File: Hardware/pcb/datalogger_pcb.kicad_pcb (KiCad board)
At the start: 2 copper layers, 123 x 86 mm, 45 parts, among them J1 Micro_SD_Card_Det2, J3 Conn_01x10_Socket, J4 Conn_01x10_Socket, J5 Conn_01x10_Socket, J6 Conn_01x04_Socket, Q1 Si2319CDS, SW1 SW_Wuerth_450301014042, SW2 SW_Push, U1 DS3231MZ, U2 SN74LVC2G00DCTR

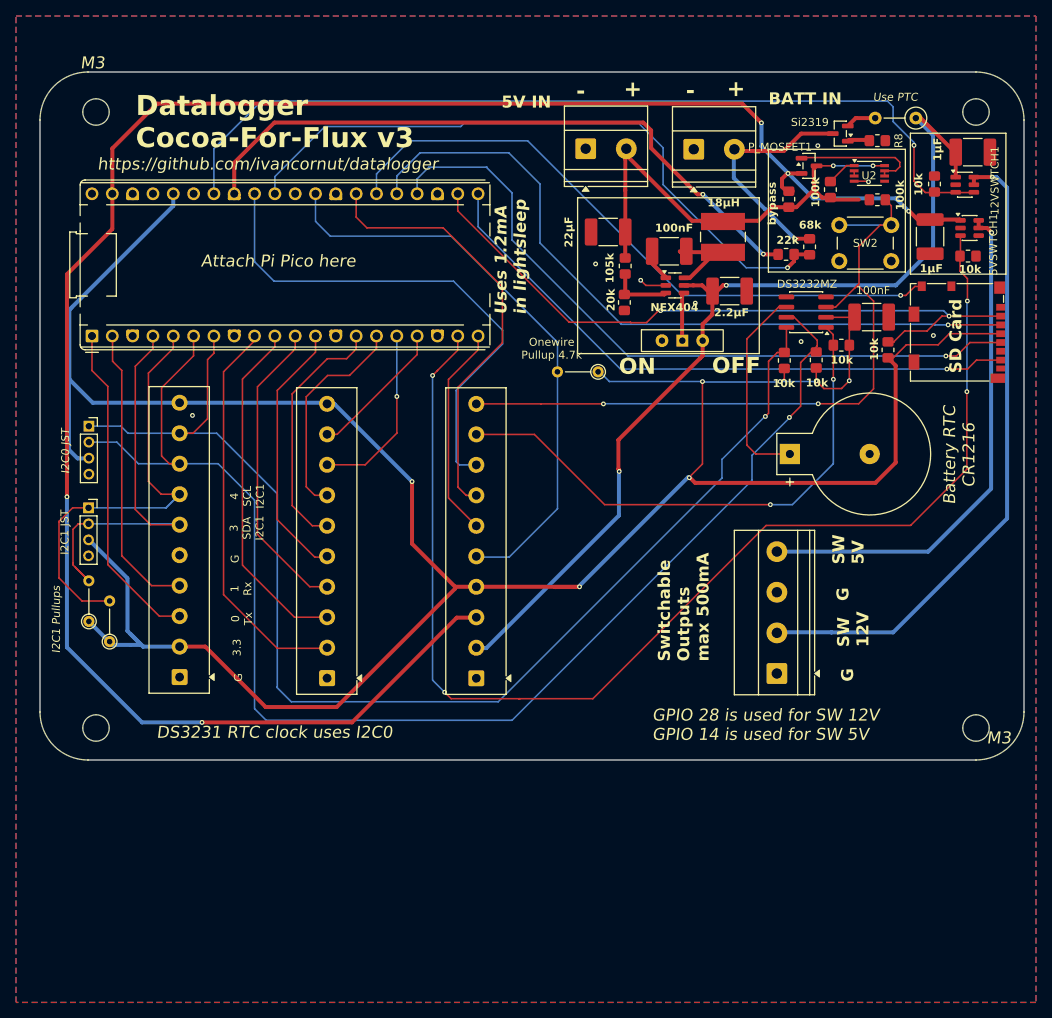
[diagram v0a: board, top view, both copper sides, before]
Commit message: Improvd pcb
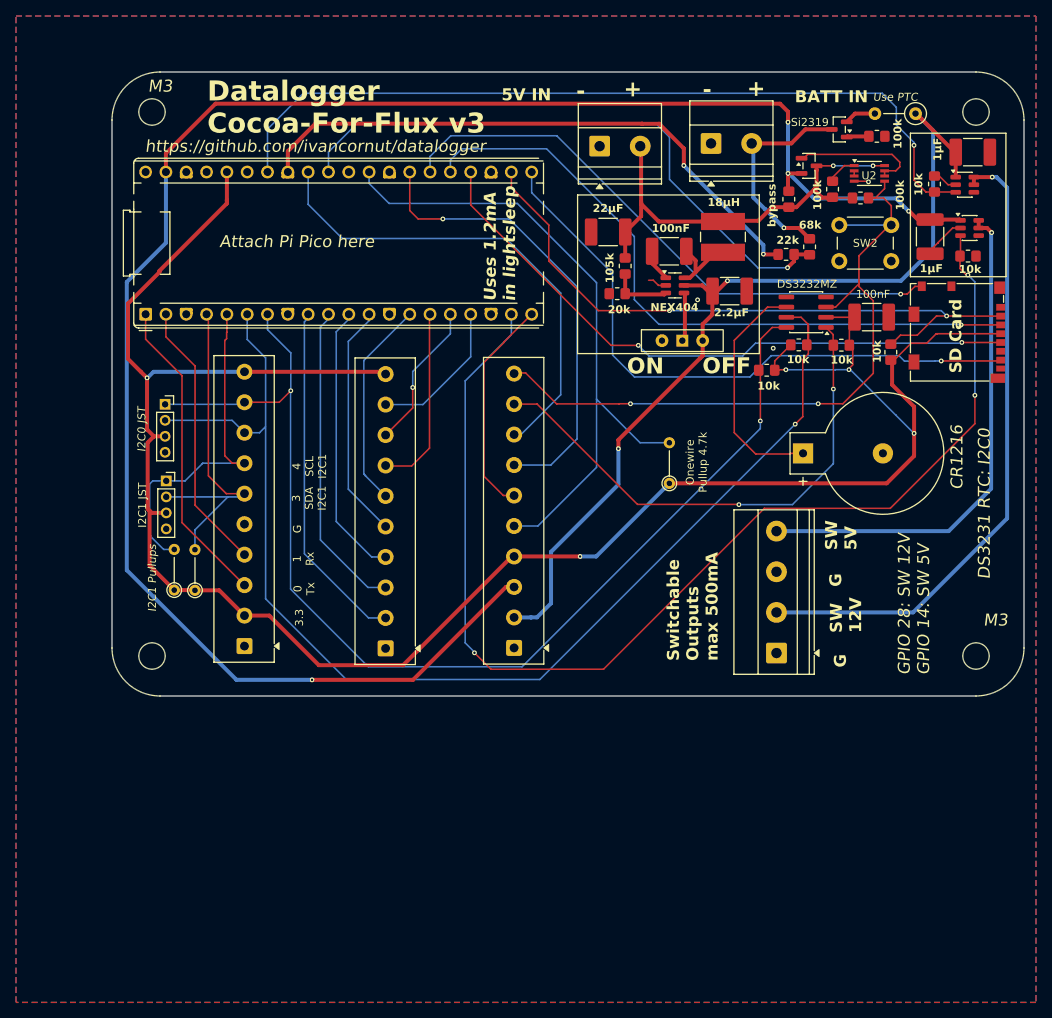
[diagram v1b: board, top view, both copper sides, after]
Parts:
- moved Pullup_One_Wire1 16.5 mm to (131.7, 86.4), turned to 90 degrees
- moved RpullupSDA1 13.8 mm to (72.4, 99.8)
- moved RpullupSCL1 10.3 mm to (69.8, 99.8)
- moved I2C1 JST 10.3 mm to (68.8, 86.1)
- moved I2C0 JST 9.91 mm to (68.6, 76.5)
- moved J5 8.99 mm to (78.6, 106.8)
- moved J3 8.20 mm to (96.2, 107.0)
- moved A1 7.23 mm to (66.2, 65.3)
- moved J4 6.05 mm to (112.3, 107.0)
- moved Rpllup1 2.89 mm to (147.8, 69.1), turned to 0 degrees
- moved J6 2.56 mm to (145.1, 107.6)
- moved Rpllup2 2.52 mm to (143.8, 72.3), turned to 180 degrees
- moved PWRIN1 2.28 mm to (136.9, 43.9)
- moved R_pullup_shtdwn1 2.12 mm to (155.6, 50.8)
- moved Alim5V1 1.77 mm to (123.0, 44.3)
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- renumbered R8 to 100k
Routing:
- net +3.3V: track 334.3 -> 265.8 mm, vias 7 -> 5
- net +5VP: track 247.6 -> 227.8 mm, vias 5 -> 4
- net /I2C0_SDA: track 170.4 -> 152.8 mm
- net /I2C0_SCL: track 157.5 -> 142.5 mm, vias 1 -> 2
- net /I2C1_SCL: track 57.6 -> 43.8 mm
- net /SCK: track 89.4 -> 78.9 mm, vias 1 -> 2
- net Net-(12VSWTCH1-EN/UVLO): track 112.3 -> 102.4 mm
- net /Data_Onewire: track 73.5 -> 82.8 mm
- net /I2C1_SDA: track 53.0 -> 44.0 mm
- net /AGND: track 82.1 -> 74.0 mm
- net Net-(5VSWTCH1-EN/UVLO): track 153.7 -> 145.7 mm, vias 4 -> 3
- net /CD: track 80.8 -> 73.2 mm
- net /MOSI: track 92.1 -> 84.6 mm
- net GND: track 5.34 -> 12.7 mm, vias 8 -> 3
- net /READ12V: track 83.1 -> 76.0 mm
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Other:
- board size 123 x 86 mm -> 114 x 78 mm
- board text added: "CR1216"
- board text added: "DS3231 RTC: I2C0"
- board text added: "GPIO 28: SW 12V GPIO 14: SW 5V"
- board text removed: "Battery RTC CR1216"
- board text removed: "DS3231 RTC clock uses I2C0"
- board text removed: "GPIO 28 is used for SW 12V GPIO 14 is used for SW 5V"
